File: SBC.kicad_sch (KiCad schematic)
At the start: 0 parts

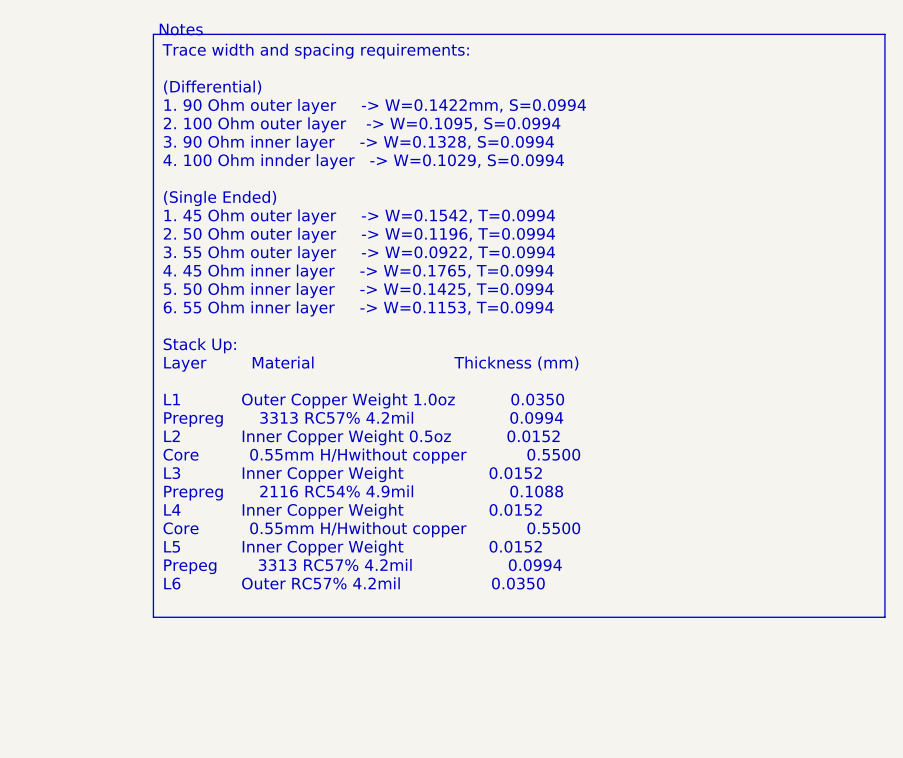
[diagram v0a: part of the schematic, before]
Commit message: Started an entire reroute
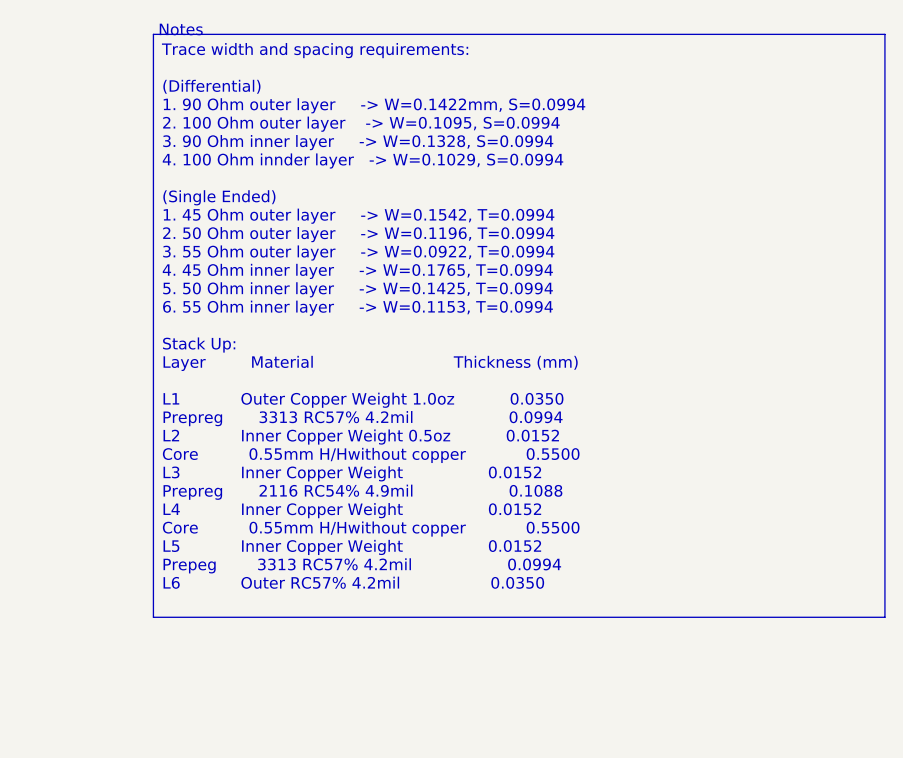
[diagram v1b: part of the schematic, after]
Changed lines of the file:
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@@
 (kicad_sch
-	(version 20231120)
+	(version 20250114)
 	(generator "eeschema")
-	(generator_version "8.0")
+	(generator_version "9.0")
 	(paper "B")
 	(title_block
@@
 		(comment 3 "Single Board Computer")
 	)
+	(text "Notes"
+		(exclude_from_sim no)
+		(at 337.058 18.796 0)
+		(effects
+			(font
+				(face "Courier New")
+				(size 1.27 1.27)
+				(color 255 255 0 1)
+			)
+		)
+	)
+	(text_box "Trace width and spacing requirements:\n\n(Differential)\n1. 90 Ohm outer layer     -> W=0.1422mm, S=0.0994\n2. 100 Ohm outer layer    -> W=0.1095, S=0.0994\n3. 90 Ohm inner layer     -> W=0.1328, S=0.0994\n4. 100 Ohm innder layer   -> W=0.1029, S=0.0994\n\n(Single Ended)\n1. 45 Ohm outer layer     -> W=0.1542, T=0.0994\n2. 50 Ohm outer layer     -> W=0.1196, T=0.0994\n3. 55 Ohm outer layer     -> W=0.0922, T=0.0994\n4. 45 Ohm inner layer     -> W=0.1765, T=0.0994\n5. 50 Ohm inner layer     -> W=0.1425, T=0.0994\n6. 55 Ohm inner layer     -> W=0.1153, T=0.0994\n\nStack Up:\nLayer         Material                            Thickness (mm)\n\nL1            Outer Copper Weight 1.0oz           0.0350\nPrepreg       3313 RC57% 4.2mil                   0.0994\nL2            Inner Copper Weight 0.5oz           0.0152\nCore          0.55mm H/Hwithout copper            0.5500\nL3            Inner Copper Weight                 0.0152\nPrepreg       2116 RC54% 4.9mil                   0.1088\nL4            Inner Copper Weight                 0.0152\nCore          0.55mm H/Hwithout copper            0.5500\nL5            Inner Copper Weight                 0.0152\nPrepeg        3313 RC57% 4.2mil                   0.0994\nL6            Outer RC57% 4.2mil                  0.0350"
+		(exclude_from_sim no)
+		(at 334.01 19.05 0)
+		(size 81.28 64.77)
+		(margins 0.9525 0.9525 0.9525 0.9525)
+		(stroke
+			(width 0)
+			(type default)
+			(color 255 255 0 1)
+		)
+		(fill
+			(type none)
+		)
+		(effects
+			(font
+				(face "Courier New")
+				(size 1.27 1.27)
+				(color 255 255 0 1)
+			)
+			(justify left top)
+		)
+	)
 	(junction
 		(at 262.89 158.75)
@@
 		)
 	)
-	(text_box "Trace width and spacing requirements:\n\n(Differential)\n1. 90 Ohm outer layer     -> W=0.1422mm, S=0.0994\n2. 100 Ohm outer layer    -> W=0.1095, S=0.0994\n3. 90 Ohm inner layer     -> W=0.1328, S=0.0994\n4. 100 Ohm innder layer   -> W=0.1029, S=0.0994\n\n(Single Ended)\n1. 45 Ohm outer layer     -> W=0.1542, T=0.0994\n2. 50 Ohm outer layer     -> W=0.1196, T=0.0994\n3. 55 Ohm outer layer     -> W=0.0922, T=0.0994\n4. 45 Ohm inner layer     -> W=0.1765, T=0.0994\n5. 50 Ohm inner layer     -> W=0.1425, T=0.0994\n6. 55 Ohm inner layer     -> W=0.1153, T=0.0994\n\nStack Up:\nLayer         Material                            Thickness (mm)\n\nL1            Outer Copper Weight 1.0oz           0.0350\nPrepreg       3313 RC57% 4.2mil                   0.0994\nL2            Inner Copper Weight 0.5oz           0.0152\nCore          0.55mm H/Hwithout copper            0.5500\nL3            Inner Copper Weight                 0.0152\nPrepreg       2116 RC54% 4.9mil                   0.1088\nL4            Inner Copper Weight                 0.0152\nCore          0.55mm H/Hwithout copper            0.5500\nL5            Inner Copper Weight                 0.0152\nPrepeg        3313 RC57% 4.2mil                   0.0994\nL6            Outer RC57% 4.2mil                  0.0350"
-		(exclude_from_sim no)
-		(at 334.01 19.05 0)
-		(size 81.28 64.77)
-		(stroke
-			(width 0)
-			(type default)
-			(color 255 255 0 1)
-		)
-		(fill
-			(type none)
-		)
-		(effects
-			(font
-				(face "Courier New")
-				(size 1.27 1.27)
-				(color 255 255 0 1)
-			)
-			(justify left top)
-		)
-	)
-	(text "Notes"
-		(exclude_from_sim no)
-		(at 337.058 18.796 0)
-		(effects
-			(font
-				(face "Courier New")
-				(size 1.27 1.27)
-				(color 255 255 0 1)
-			)
-		)
-	)
 	(netclass_flag ""
 		(length 0.0254)
@@
 		(at 281.94 38.1)
 		(size 27.94 104.14)
+		(exclude_from_sim no)
+		(in_bom yes)
+		(on_board yes)
+		(dnp no)
 		(fields_autoplaced yes)
 		(stroke
@@
 		(at 179.07 38.1)
 		(size 49.53 104.14)
+		(exclude_from_sim no)
+		(in_bom yes)
+		(on_board yes)
+		(dnp no)
 		(fields_autoplaced yes)
 		(stroke
@@
 		(at 234.95 166.37)
 		(size 85.09 26.67)
+		(exclude_from_sim no)
+		(in_bom yes)
+		(on_board yes)
+		(dnp no)
 		(fields_autoplaced yes)
 		(stroke
@@
 		(at 105.41 106.68)
 		(size 41.91 36.83)
+		(exclude_from_sim no)
+		(in_bom yes)
+		(on_board yes)
+		(dnp no)
 		(fields_autoplaced yes)
 		(stroke
@@
 		(at 105.41 38.1)
 		(size 41.91 59.69)
+		(exclude_from_sim no)
+		(in_bom yes)
+		(on_board yes)
+		(dnp no)
 		(fields_autoplaced yes)
 		(stroke
@@
 		)
 	)
+	(embedded_fonts no)
 )
